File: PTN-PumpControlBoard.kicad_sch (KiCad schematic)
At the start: 14 parts, among them IC1 ADT7470ARQZ-REEL7, IC2 ADS131M03QPWRQ1, J1 Conn_01x04, U1 PeripheralSOM, U2 ST7735R

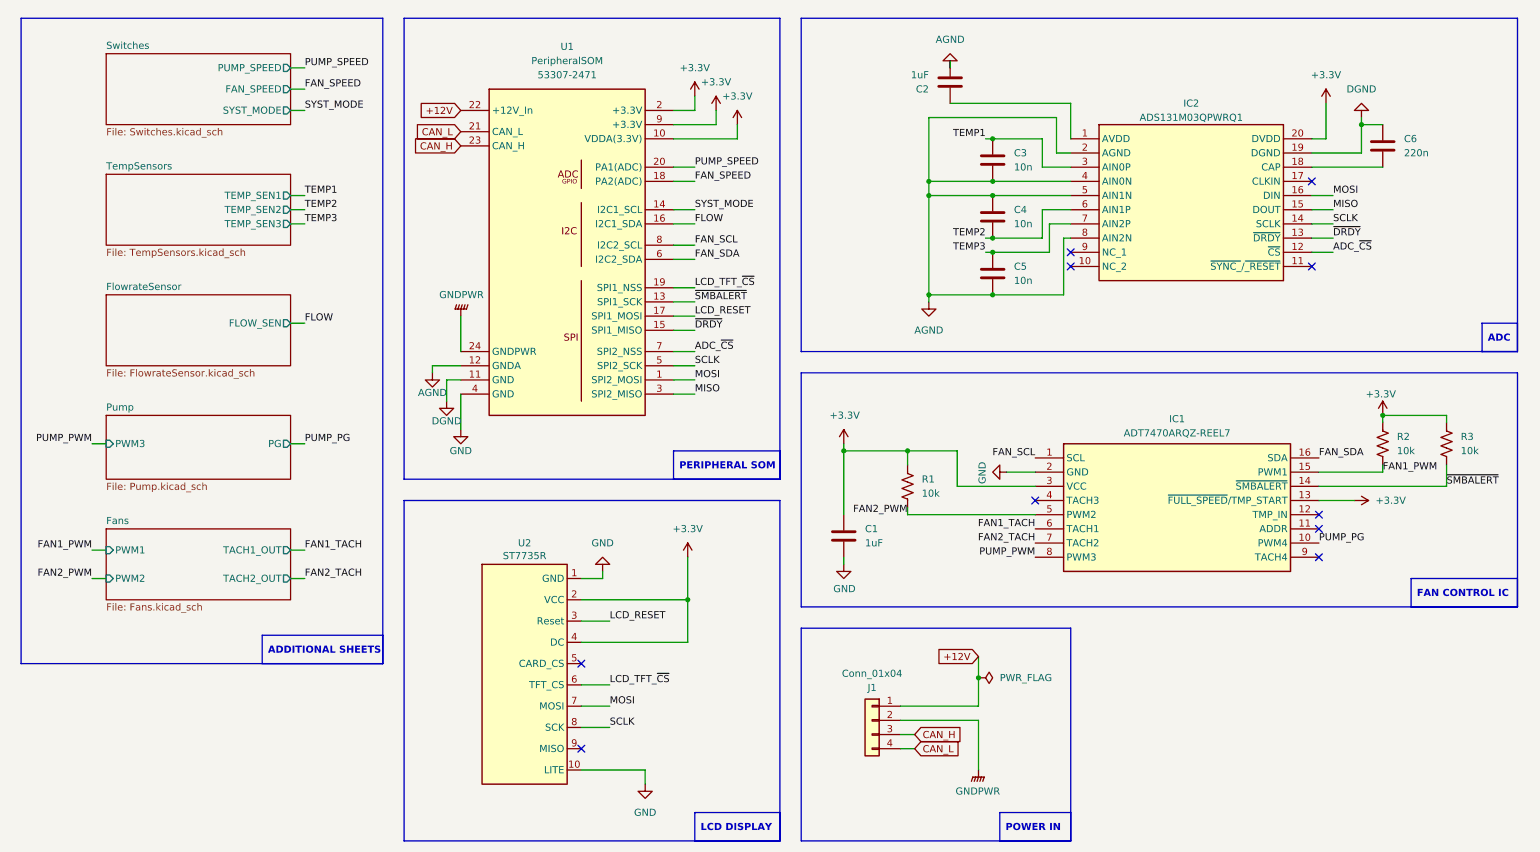
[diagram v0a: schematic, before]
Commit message: Initial schematic design with 2 temp, 1 flow, 1 pump
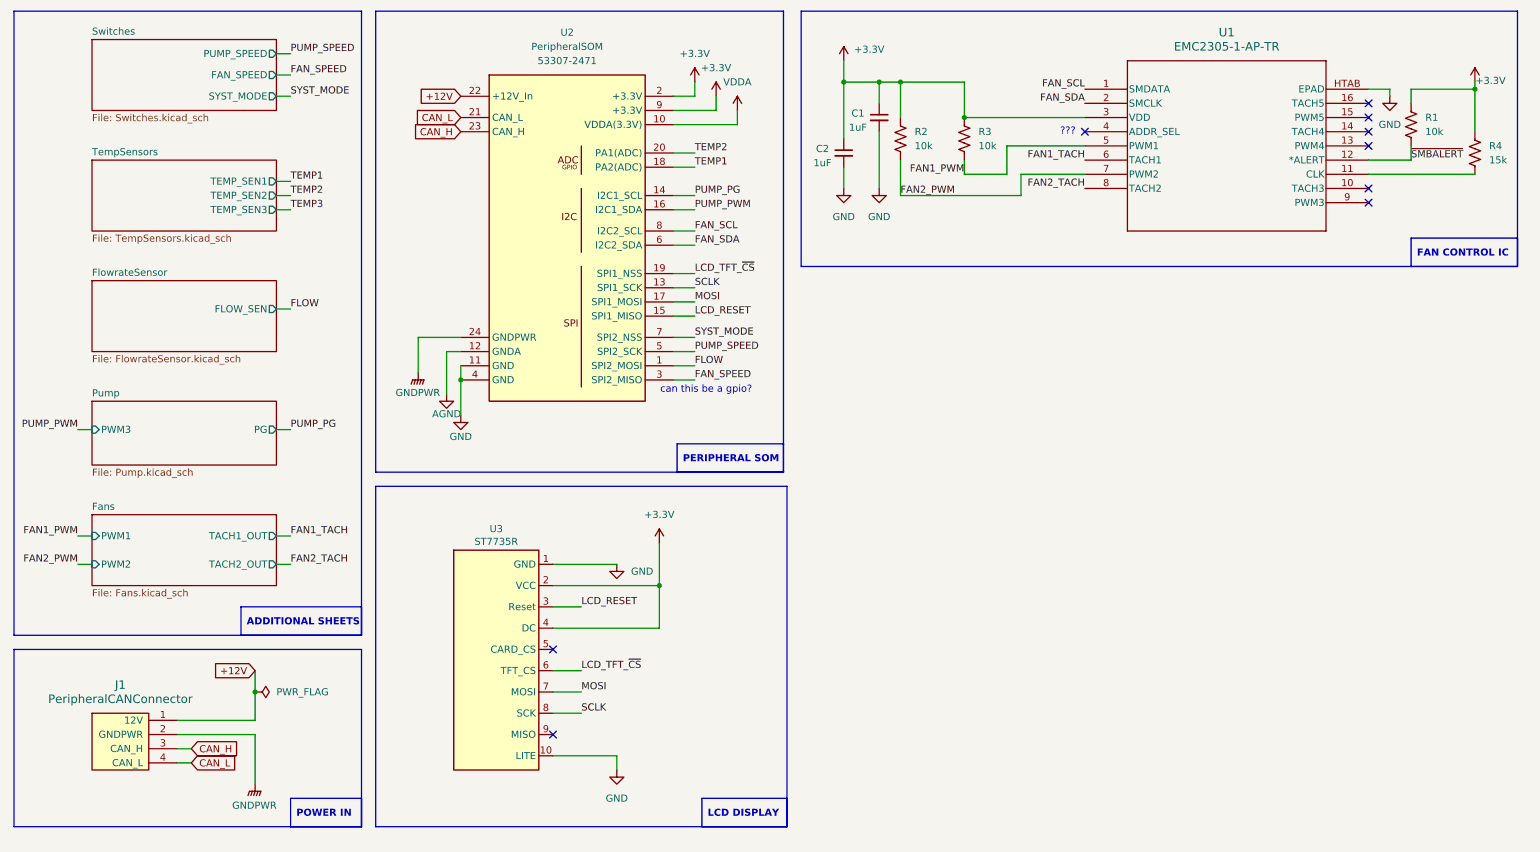
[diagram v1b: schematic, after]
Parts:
- removed C1, C2: 1uF, Capacitor_SMD:C_0805_2012Metric, symbol Device:C
- removed C3, C4, C5: 10n, Capacitor_SMD:C_0805_2012Metric, symbol Device:C
- removed C6: 220n, Capacitor_SMD:C_0805_2012Metric, symbol Device:C
- removed IC1: ADT7470ARQZ-REEL7, Package_SO:QSOP-16_3.9x4.9mm_P0.635mm, symbol utsvt-chips:ADT7470ARQZ
- removed IC2: ADS131M03QPWRQ1, SOP65P640X120-20N, symbol ADS131M03QPWRQ1:ADS131M03QPWRQ1
- removed J1: Conn_01x04, UTSVT_Connectors:Molex_MicroFit3.0_1x4xP3.00mm_PolarizingPeg_Vertical, symbol Connector_Generic:Conn_01x04
- removed U1: PeripheralSOM, UTSVT_Special:PeripheralSOM, symbol utsvt-misc:PeripheralSOM
- added C1, C2: 1uF, Capacitor_SMD:C_0805_2012Metric, symbol Device:C_Small
- added J1: PeripheralCANConnector, UTSVT_Connectors:Molex_MicroFit3.0_1x4xP3.00mm_PolarizingPeg_Vertical, symbol utsvt-connectors:PeripheralCANConnector
- added R4: 15k, Resistor_SMD:R_0805_2012Metric, symbol Device:R_US
- added U1: EMC2305-1-AP-TR, FanControl:QFN16_4x4MC_MCH, symbol 2024-11-02_21-04-42:EMC2305-1-AP-TR
- added U2: PeripheralSOM, UTSVT_Special:PeripheralSOM, symbol utsvt-misc:PeripheralSOM
- renumbered U2 to U3
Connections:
- net +12V: now also J1.1 (12V), U2.22 (+12V_In)
- net +3.3V: now also R1.2, C1.1, C2.1, R4.2, U1.3 (VDD), U2.2 (+3.3V), U2.9 (+3.3V); no longer R1.1
- net AGND: now also U2.12 (GNDA)
- net CAN_H: now also J1.3 (CAN_H), U2.23 (CAN_H)
- net CAN_L: now also J1.4 (CAN_L), U2.21 (CAN_L)
- net FAN1_PWM: now also R3.1, U1.5 (PWM1); no longer R2.1
- net FAN1_TACH: now also U1.6 (TACH1)
- net FAN2_PWM: now also R2.1, U1.7 (PWM2); no longer R1.2
- net FAN2_TACH: now also U1.8 (TACH2)
- net FAN_SCL: now also U1.1 (SMDATA), U2.8 (I2C2_SCL)
- net FAN_SDA: now also U1.2 (SMCLK), U2.6 (I2C2_SDA)
- net FAN_SPEED: now also U2.3 (SPI2_MISO)
- net FLOW: now also U2.1 (SPI2_MOSI)
- net GND: now also C1.2, C2.2, U1.HTAB (EPAD), U2.11 (GND), U2.4 (GND)
- net GNDPWR: now also J1.2 (GNDPWR), U2.24 (GNDPWR)
- net LCD_RESET: now also U2.15 (SPI1_MISO)
- net LCD_TFT_~{CS}: now also U2.19 (SPI1_NSS)
- net MOSI: now also U2.17 (SPI1_MOSI)
- net PUMP_PG: now also U2.14 (I2C1_SCL)
- net PUMP_PWM: now also U2.16 (I2C1_SDA)
- net PUMP_SPEED: now also U2.5 (SPI2_SCK)
- net SCLK: now also U2.13 (SPI1_SCK)
- net SYST_MODE: now also U2.7 (SPI2_NSS)
- net TEMP1: now also U2.18 (PA2(ADC))
- net TEMP2: now also U2.20 (PA1(ADC))
- net ~{SMBALERT}: now also R1.1, U1.12 (*ALERT); no longer R3.1
- new net: R4.1, U1.11 (CLK)
- new net VDDA: U2.10 (VDDA(3.3V))
- no-connect marks 10 -> 9
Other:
- note added: "???"
- note added: "can this be a gpio?"
- moved on the sheet: U3
